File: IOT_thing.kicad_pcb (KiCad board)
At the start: 4 copper layers, 100 x 100 mm, 64 parts, among them J1 USB_C_Receptacle_USB2.0_16P, J2 Conn_01x04, J3 Screw_Terminal_01x03, J4 Screw_Terminal_01x08, J5 Screw_Terminal_01x02, J6 Conn_02x05_Odd_Even, K1 RT314A05, Q1 UMH3N, Q2 UMH3N, Q3 BC817, SW1 SW_SPST, U1 ESP32-WROOM-32D, U2 USBLC6-2P6, U3 CP2104, U4 Si7021-A20, U5 74AHCT245, U6 TLV117LV-3.3V

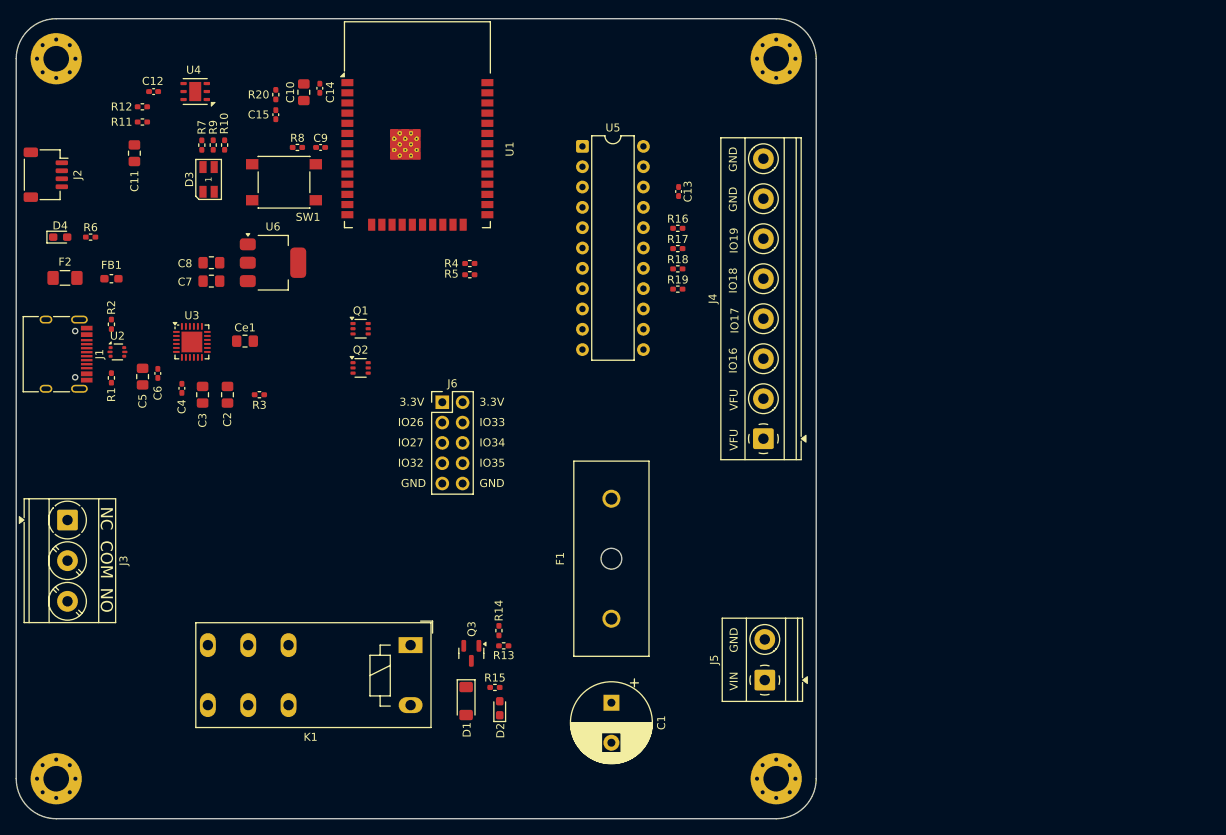
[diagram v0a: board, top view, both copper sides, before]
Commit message: Finalised the project
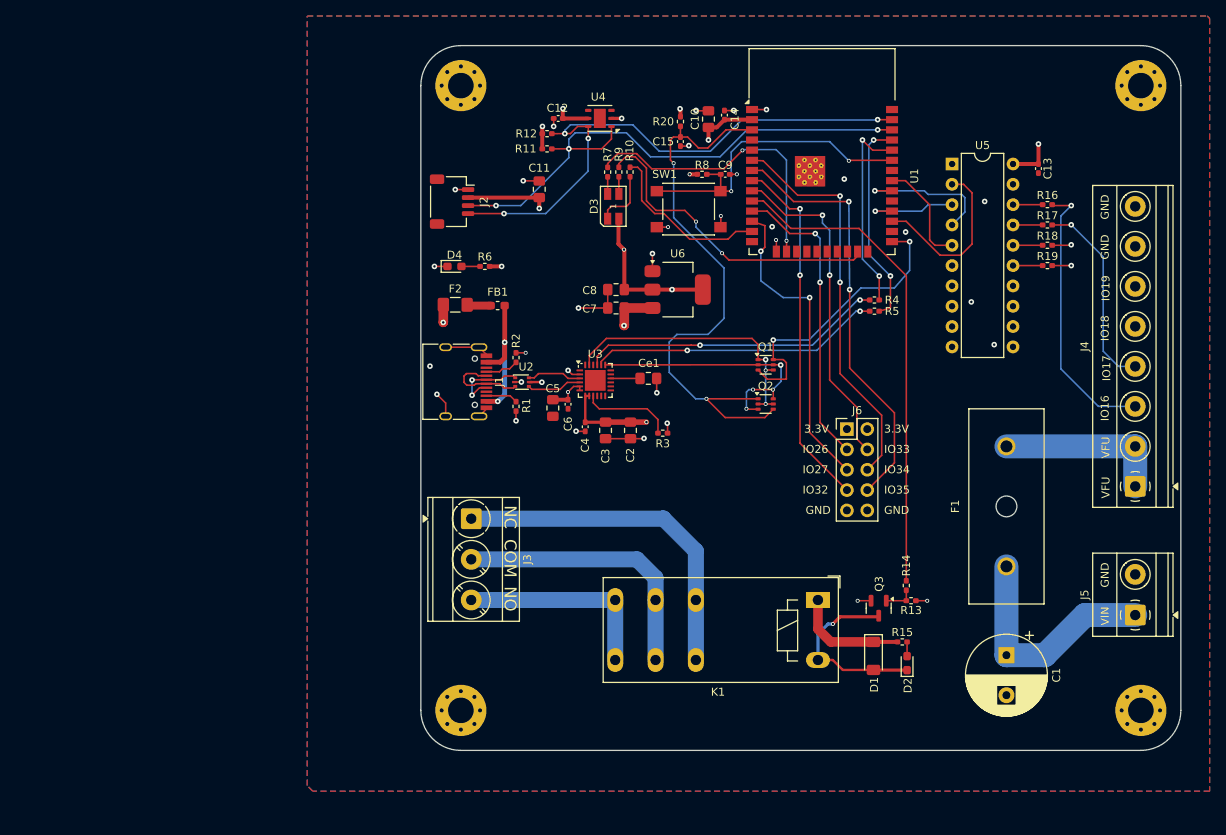
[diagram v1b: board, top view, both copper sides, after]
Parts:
- U2: footprint Package_TO_SOT_SMD:SOT-666 -> iot-thing_Library_11:SOT-666
- U5: footprint Package_DIP:DIP-22_W7.62mm -> iot-thing_Library_11:DIP-20_W7.62mm
- moved C5 51.4 mm to (125.7, 96.2)
- moved C6 51.4 mm to (127.6, 95.7)
- moved H3 51.3 mm to (114.2, 134.0)
- moved R15 51.2 mm to (169.4, 125.4)
- moved R14 51.2 mm to (169.9, 118.3)
- moved D2 51.2 mm to (170.0, 128.1)
- moved Q3 51.2 mm to (166.4, 121.2)
- moved R13 51.2 mm to (170.5, 120.2)
- moved D1 51.2 mm to (165.8, 127.2)
- moved K1 51.2 mm to (158.8, 120.2)
- moved J2 50.9 mm to (113.1, 70.4)
- moved R7 50.8 mm to (132.5, 66.7)
- moved Q1 50.8 mm to (152.3, 90.8)
- moved Q2 50.8 mm to (152.3, 95.7)
- moved R9 50.8 mm to (133.9, 66.7)
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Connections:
- C15 pad 1: Net-(C15-Pad1) -> /EN
- H3 pad 1: GND -> unconnected-(H3-Pad1)_4
- Q2 pad 1: +3.3V -> /EN
- Q2 pad 4: +3.3V -> /EN
- R20 pad 2: Net-(C15-Pad1) -> /EN
- U1 pad 3: +3.3V -> /EN
- U1 pad 34: /TX -> /RX
- U1 pad 35: /RX -> /TX
- U2 pad 1: Net-(U3-D-) -> Net-(J1-D+-PadA6)
- U2 pad 4: Net-(J1-D+-PadA6) -> Net-(U3-D-)
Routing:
- net +5V: track 0.00 -> 211.0 mm, vias 0 -> 5
- net +3.3V: track 0.00 -> 155.0 mm, vias 0 -> 9
- net /EN: track 0.00 -> 72.4 mm, vias 0 -> 2
- net /SCL: track 0.00 -> 72.4 mm, vias 0 -> 4
- net /SDA: track 0.00 -> 70.4 mm, vias 0 -> 3
- net /RELAY: track 0.00 -> 61.3 mm
- net /GPIO35: track 0.00 -> 53.5 mm, vias 0 -> 2
- net GND: track 0.00 -> 52.9 mm, vias 0 -> 31
- net /GPIO34: track 0.00 -> 49.9 mm, vias 0 -> 2
- net /GPIO32: track 0.00 -> 45.0 mm, vias 0 -> 2
- net Net-(J3-Pin_1): track 0.00 -> 43.4 mm
- net /GPIO33: track 0.00 -> 41.7 mm, vias 0 -> 2
- net /SW: track 0.00 -> 39.7 mm, vias 0 -> 2
- net /LED_G: track 0.00 -> 39.6 mm, vias 0 -> 2
- net /GPIO27: track 0.00 -> 39.0 mm, vias 0 -> 2
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- added copper zone on B.Cu, net GND
- added copper zone on F.Cu, net GND
- added copper zone on In1.Cu, net GND
- added copper zone on In2.Cu, net GND
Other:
- board size 100 x 100 mm -> 95 x 88.1 mm
